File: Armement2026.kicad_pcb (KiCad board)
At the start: 2 copper layers, 87.5 x 77.5 mm, 31 parts, among them J1 Screw_Terminal_01x02, J10 Screw_Terminal_01x02, J11 Screw_Terminal_01x02, J2 Screw_Terminal_01x02, J3 Screw_Terminal_01x02, J4 Screw_Terminal_01x02, J5 Screw_Terminal_01x02, J6 Screw_Terminal_01x02, J7 Screw_Terminal_01x02, J8 Screw_Terminal_01x02, J9 Screw_Terminal_01x02, Q1 NTR4101PT1G, Q2 NTR4101PT1G, SW1 SW_Nidec_CAS-120A1, SW2 SW_Nidec_CAS-120A1, SW3 SW_Nidec_CAS-120A1, SW4 SW_Nidec_CAS-120A1, U1 LDO_4v2-MIC5209-4.2YS-TR

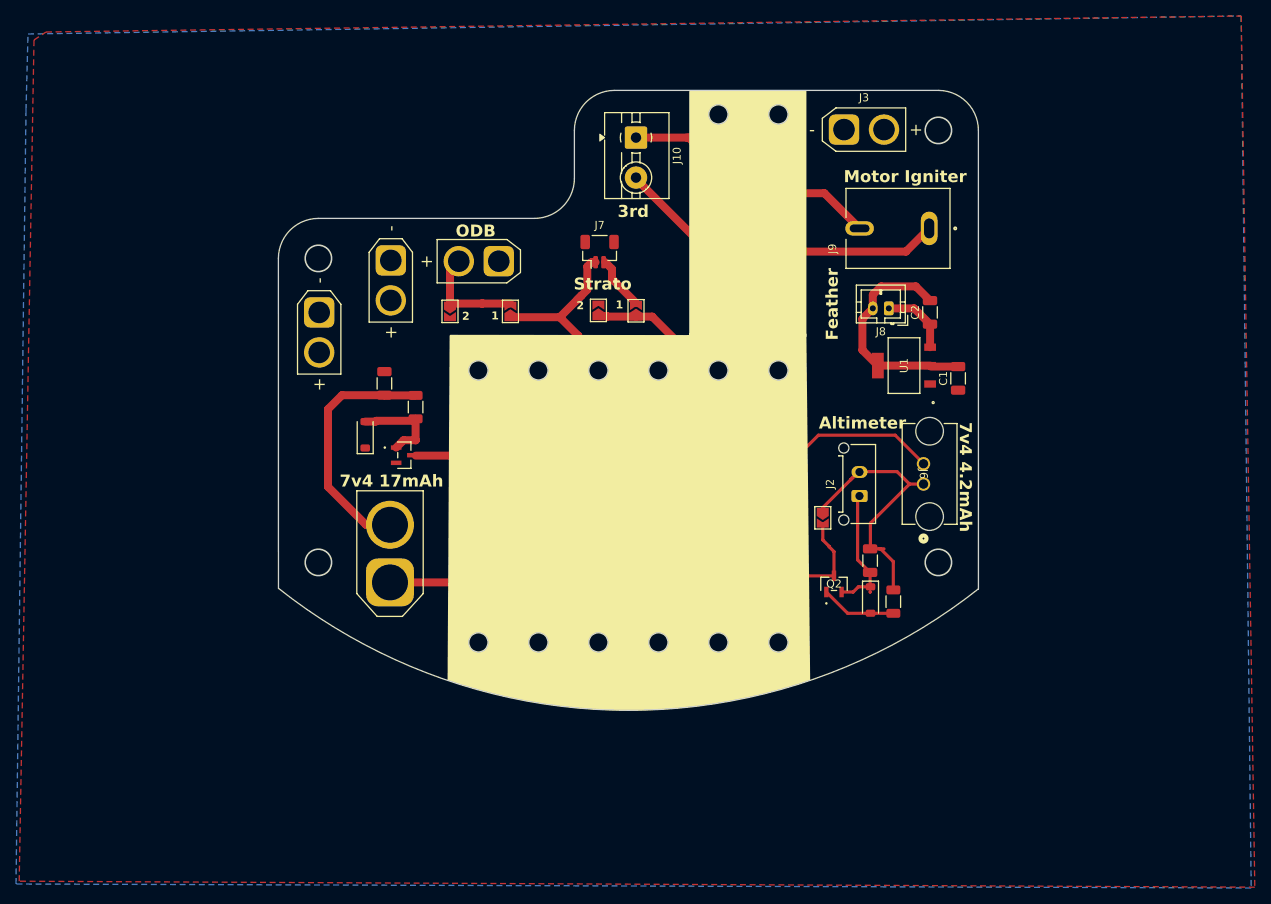
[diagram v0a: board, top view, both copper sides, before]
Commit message: wtf did I just do
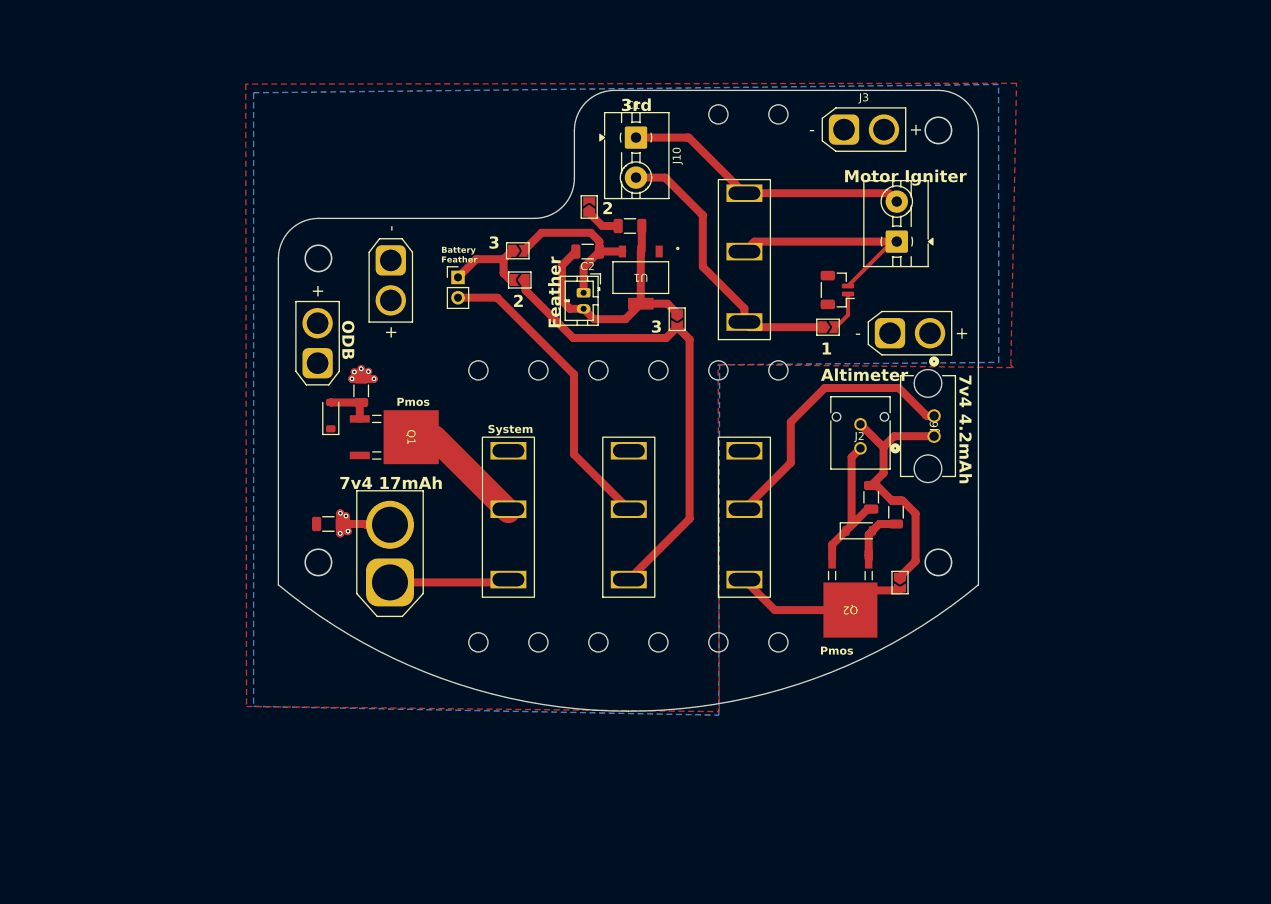
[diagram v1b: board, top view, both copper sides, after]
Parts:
- added G***: LOGO, LOGO, F.Cu at (100.2, 157.6)
- added J12: Screw_Terminal_01x02, TerminalBlock:TerminalBlock_MaiXu_MX126-5.0-02P_1x02_P5.00mm, F.Cu at (133.3, 102.9)
- added JP6: SolderJumper_2_Open, Jumper:SolderJumper-2_P1.3mm_Open_TrianglePad1.0x1.5mm, F.Cu at (86.2, 107.7)
- J2: footprint Connector_Molex:Molex_Micro-Fit_3.0_43650-0215_1x02_P3.00mm_Vertical -> 3mm header 2x1:CONN_SD-44067-001_02_MOL
- J7: footprint Connector_JST:JST_SH_BM02B-SRSS-TB_1x02-1MP_P1.00mm_Vertical -> Connector_PinHeader_2.54mm:PinHeader_1x02_P2.54mm_Vertical
- J9: footprint RCJ_054:CUI_RCJ-054 -> Connector_JST:JST_SH_BM02B-SRSS-TB_1x02-1MP_P1.00mm_Vertical
- Q1, Q2: value NTR4101PT1G -> DMP10H400SK3-13; footprint NTR4101PT1G:SOT-23-3_1P4X3P040_ONS -> footprints3:TO252-DPAK-DMP10H400SK3_DIO
- moved J4 71.4 mm to (132.4, 114.3), turned to 0 degrees
- moved C1 45.2 mm to (100.0, 101.0), turned to 0 degrees
- moved C2 43.5 mm to (94.7, 104.2), turned to 180 degrees
- moved J8 38.2 mm to (94.2, 109.3), turned to -90 degrees
- moved U1 34.7 mm to (101.3, 107.4), turned to 180 degrees
- moved J5 26.0 mm to (60.9, 118.1), turned to 90 degrees
- moved JP4 24.1 mm to (124.7, 113.6), turned to 0 degrees
- moved JP2 21.7 mm to (94.8, 98.6), turned to 90 degrees
- moved JP5 20.9 mm to (105.8, 112.6), turned to -90 degrees
- moved C8 18.9 mm to (62.2, 138.2), turned to 0 degrees
- moved J7 18.0 mm to (78.5, 107.4)
- moved JP1 12.6 mm to (133.7, 145.5)
- moved JP3 12.5 mm to (85.9, 104.0), turned to 0 degrees
- moved PWR_R2 11.2 mm to (133.2, 136.7)
- moved J9 9.81 mm to (125.9, 109.0)
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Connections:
- C1 pad 1: 7v4 -> Net-(JP2-A)
- J5 pad 2: Net-(J5-Pin_2) -> 7v4
- J6 pad 1: Net-(J2-Pin_2) -> Net-(J6-Pin_1)
- J6 pad 2: Net-(J6-Pin_2) -> Net-(J2-Pin_2)
- J9 pad 2: Net-(J10-Pin_1) -> Net-(J12-Pin_1)
- JP2 pad 1: Net-(J5-Pin_2) -> Net-(JP2-A)
- JP3 pad 1: Net-(JP3-A) -> Net-(J7-Pin_1)
- JP3 pad 2: 7v4 -> Net-(J8-Pin_1)
- JP4 pad 1: Net-(JP3-A) -> Net-(J10-Pin_2)
- JP4 pad 2: Net-(J7-Pin_2) -> Net-(J9-Pin_1)
- JP5 pad 1: Net-(J7-Pin_1) -> GND
- JP5 pad 2: Net-(J5-Pin_2) -> Net-(JP5-B)
- SW2 pad 1: Net-(J7-Pin_1) -> Net-(JP5-B)
- SW2 pad 2: Net-(JP3-A) -> Net-(J7-Pin_2)
- SW3 pad 2: Net-(J6-Pin_2) -> Net-(J6-Pin_1)
- SW4 pad 2: Net-(J9-Pin_1) -> Net-(J12-Pin_1)
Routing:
- net Net-(JP5-B): track 0.00 -> 58.6 mm
- net Net-(J7-Pin_1): track 52.4 -> 11.3 mm
- net Net-(JP3-A): track 35.8 -> 0.00 mm
- net Net-(J6-Pin_1): track 0.00 -> 34.4 mm
- net Net-(J7-Pin_2): track 6.69 -> 38.3 mm
- net Net-(J12-Pin_1): track 0.00 -> 28.0 mm
- net Net-(J6-Pin_2): track 27.7 -> 0.00 mm
- net Net-(J9-Pin_1): track 24.3 -> 4.78 mm
- net Net-(J5-Pin_2): track 13.7 -> 0.00 mm
- net Net-(J10-Pin_2): track 23.7 -> 35.8 mm
- net Net-(J8-Pin_1): track 8.85 -> 20.9 mm
- net GND: track 59.3 -> 51.3 mm, vias 0 -> 9
- net Net-(DZ1-A): track 12.0 -> 5.93 mm
- net Net-(JP2-A): track 0.00 -> 4.31 mm
- net Net-(JP1-B): track 18.3 -> 22.0 mm
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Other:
- board size 87.5 x 77.5 mm -> 87.5 x 77.6 mm
- board text added: "3"
- board text added: "Battery Feather"
- board text added: "Pmos"
- board text added: "System"
- board text removed: "Option 1: Solder this option to use the ODB as the third flight computer. Option 2: Solder this option to use the ODB as the second flight computer (without the Stratologger)."
- board text removed: "Strato"
